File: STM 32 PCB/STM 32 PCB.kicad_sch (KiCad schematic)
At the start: 0 parts

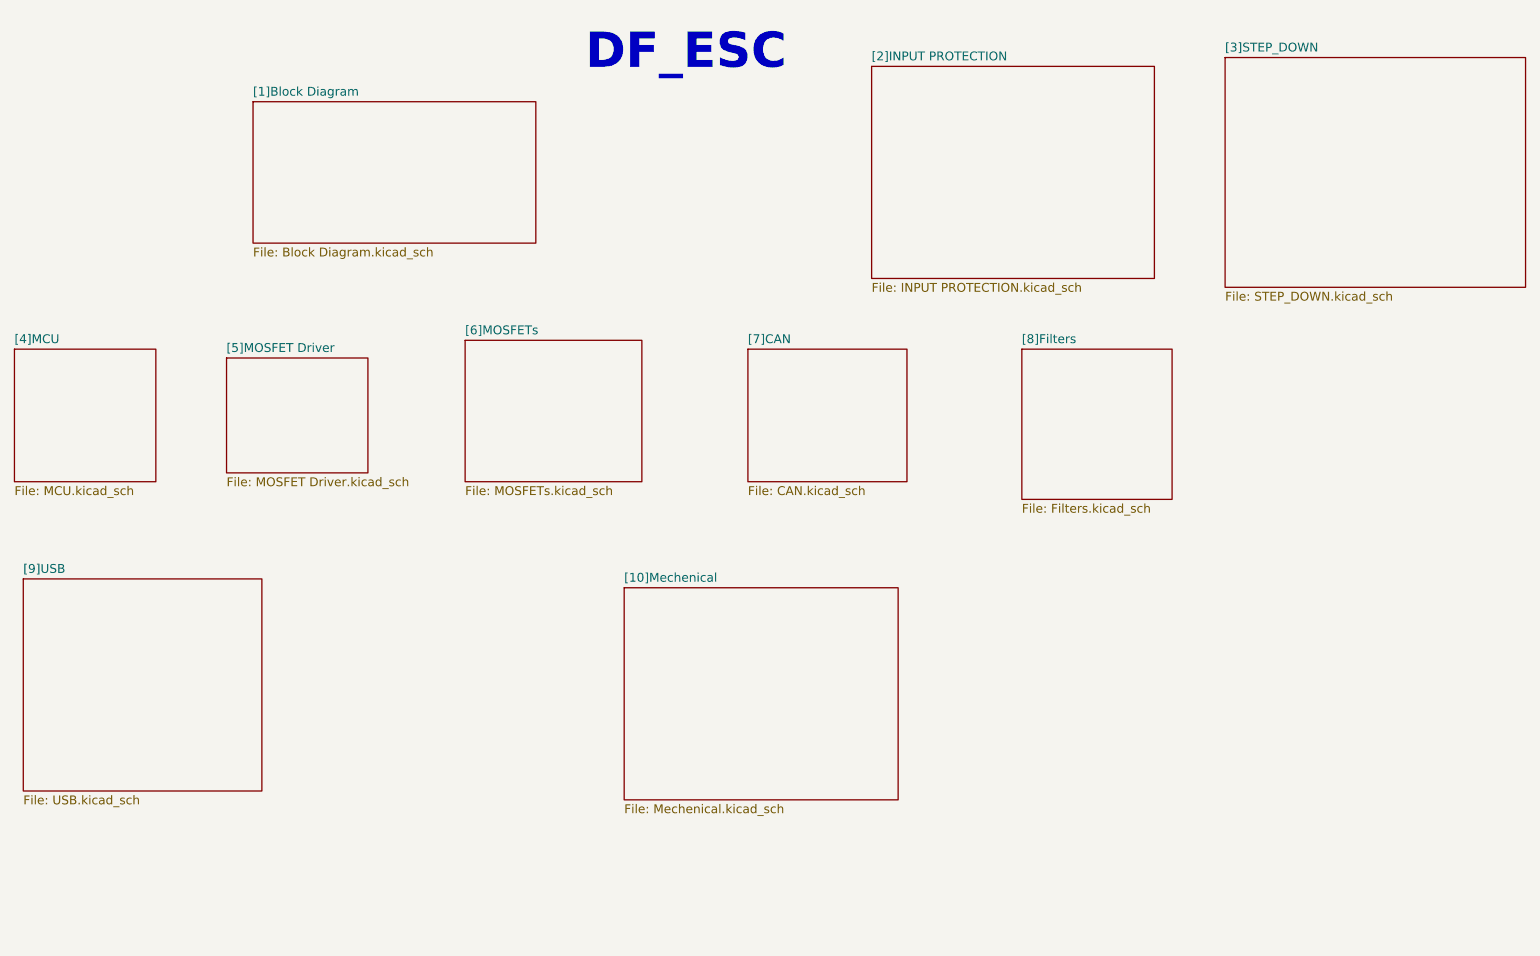
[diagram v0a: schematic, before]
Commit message: 11 Dec
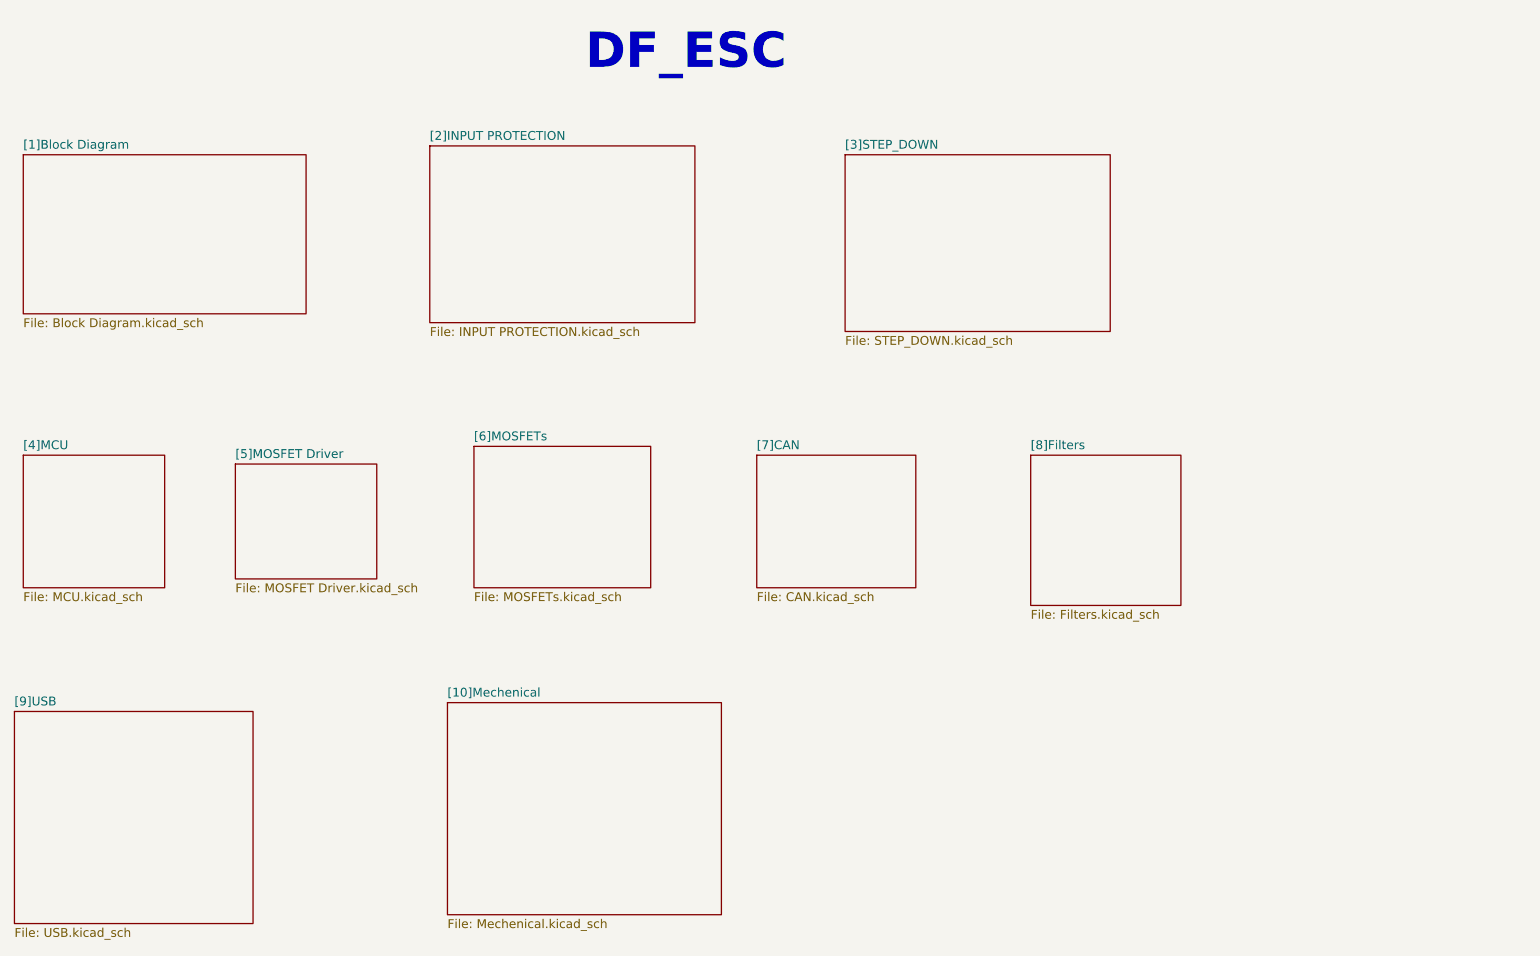
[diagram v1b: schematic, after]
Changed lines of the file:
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@@
 	)
 	(sheet
-		(at 119.38 60.96)
+		(at 120.65 76.2)
 		(size 25.4 20.32)
 		(fields_autoplaced yes)
@@
 		)
 		(property "Sheetname" "[6]MOSFETs"
-			(at 119.38 60.2484 0)
+			(at 120.65 75.4884 0)
 			(effects
 				(font
@@
 		)
 		(property "Sheetfile" "MOSFETs.kicad_sch"
-			(at 119.38 81.8646 0)
+			(at 120.65 97.1046 0)
 			(effects
 				(font
@@
 	)
 	(sheet
-		(at 88.9 26.67)
-		(size 40.64 20.32)
+		(at 55.88 34.29)
+		(size 40.64 22.86)
 		(fields_autoplaced yes)
 		(stroke
@@
 		)
 		(property "Sheetname" "[1]Block Diagram"
-			(at 88.9 25.9584 0)
+			(at 55.88 33.5784 0)
 			(effects
 				(font
@@
 		)
 		(property "Sheetfile" "Block Diagram.kicad_sch"
-			(at 88.9 47.5746 0)
+			(at 55.88 57.7346 0)
 			(effects
 				(font
@@
 	)
 	(sheet
-		(at 85.09 63.5)
+		(at 86.36 78.74)
 		(size 20.32 16.51)
 		(fields_autoplaced yes)
@@
 		)
 		(property "Sheetname" "[5]MOSFET Driver"
-			(at 85.09 62.7884 0)
+			(at 86.36 78.0284 0)
 			(effects
 				(font
@@
 		)
 		(property "Sheetfile" "MOSFET Driver.kicad_sch"
-			(at 85.09 80.5946 0)
+			(at 86.36 95.8346 0)
 			(effects
 				(font
@@
 	)
 	(sheet
-		(at 142.24 96.52)
+		(at 116.84 113.03)
 		(size 39.37 30.48)
 		(fields_autoplaced yes)
@@
 		)
 		(property "Sheetname" "[10]Mechenical"
-			(at 142.24 95.8084 0)
+			(at 116.84 112.3184 0)
 			(effects
 				(font
@@
 		)
 		(property "Sheetfile" "Mechenical.kicad_sch"
-			(at 142.24 127.5846 0)
+			(at 116.84 144.0946 0)
 			(effects
 				(font
@@
 	)
 	(sheet
-		(at 228.6 20.32)
-		(size 43.18 33.02)
+		(at 173.99 34.29)
+		(size 38.1 25.4)
 		(fields_autoplaced yes)
 		(stroke
@@
 		)
 		(property "Sheetname" "[3]STEP_DOWN"
-			(at 228.6 19.6084 0)
+			(at 173.99 33.5784 0)
 			(effects
 				(font
@@
 		)
 		(property "Sheetfile" "STEP_DOWN.kicad_sch"
-			(at 228.6 53.9246 0)
+			(at 173.99 60.2746 0)
 			(effects
 				(font
@@
 	)
 	(sheet
-		(at 199.39 62.23)
+		(at 200.66 77.47)
 		(size 21.59 21.59)
 		(fields_autoplaced yes)
@@
 		)
 		(property "Sheetname" "[8]Filters"
-			(at 199.39 61.5184 0)
+			(at 200.66 76.7584 0)
 			(effects
 				(font
@@
 		)
 		(property "Sheetfile" "Filters.kicad_sch"
-			(at 199.39 84.4046 0)
+			(at 200.66 99.6446 0)
 			(effects
 				(font
@@
 	)
 	(sheet
-		(at 55.88 95.25)
+		(at 54.61 114.3)
 		(size 34.29 30.48)
 		(fields_autoplaced yes)
@@
 		)
 		(property "Sheetname" "[9]USB"
-			(at 55.88 94.5384 0)
+			(at 54.61 113.5884 0)
 			(effects
 				(font
@@
 		)
 		(property "Sheetfile" "USB.kicad_sch"
-			(at 55.88 126.3146 0)
+			(at 54.61 145.3646 0)
 			(effects
 				(font
@@
 	)
 	(sheet
-		(at 160.02 62.23)
+		(at 161.29 77.47)
 		(size 22.86 19.05)
 		(fields_autoplaced yes)
@@
 		)
 		(property "Sheetname" "[7]CAN"
-			(at 160.02 61.5184 0)
+			(at 161.29 76.7584 0)
 			(effects
 				(font
@@
 		)
 		(property "Sheetfile" "CAN.kicad_sch"
-			(at 160.02 81.8646 0)
+			(at 161.29 97.1046 0)
 			(effects
 				(font
@@
 	)
 	(sheet
-		(at 54.61 62.23)
+		(at 55.88 77.47)
 		(size 20.32 19.05)
 		(fields_autoplaced yes)
@@
 		)
 		(property "Sheetname" "[4]MCU"
-			(at 54.61 61.5184 0)
+			(at 55.88 76.7584 0)
 			(effects
 				(font
@@
 		)
 		(property "Sheetfile" "MCU.kicad_sch"
-			(at 54.61 81.8646 0)
+			(at 55.88 97.1046 0)
 			(effects
 				(font
@@
 	)
 	(sheet
-		(at 177.8 21.59)
-		(size 40.64 30.48)
+		(at 114.3 33.02)
+		(size 38.1 25.4)
 		(fields_autoplaced yes)
 		(stroke
@@
 		)
 		(property "Sheetname" "[2]INPUT PROTECTION"
-			(at 177.8 20.8784 0)
+			(at 114.3 32.3084 0)
 			(effects
 				(font
@@
 		)
 		(property "Sheetfile" "INPUT PROTECTION.kicad_sch"
-			(at 177.8 52.6546 0)
-			(effects
-				(font
+			(at 114.3 59.0046 0)
+			(effects
+				(font
